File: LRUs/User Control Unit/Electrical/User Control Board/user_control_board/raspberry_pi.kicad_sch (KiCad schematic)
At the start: 2 parts, among them SW1 SW_SPDT

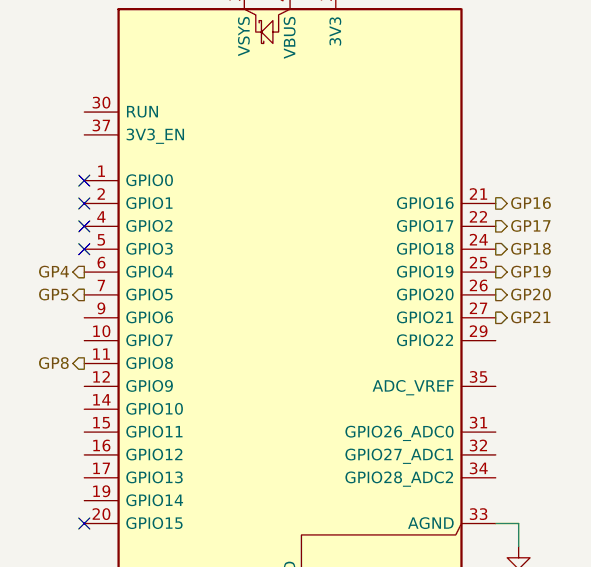
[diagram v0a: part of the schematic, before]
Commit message: DAC added Removed unnecessary modules.
Need to make custom footprint for dac.
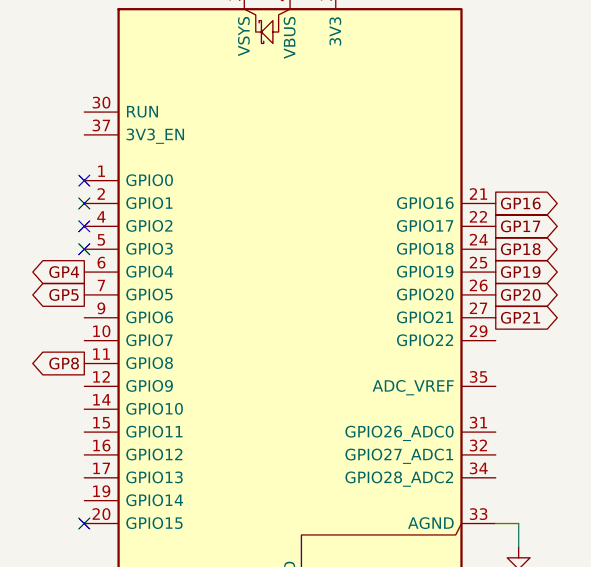
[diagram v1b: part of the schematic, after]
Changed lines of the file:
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@@
 		)
 	)
-	(hierarchical_label "GP19"
+	(global_label "GP18"
+		(shape output)
+		(at 168.91 88.9 0)
+		(fields_autoplaced yes)
+		(effects
+			(font
+				(size 1.27 1.27)
+			)
+			(justify left)
+		)
+		(property "Intersheetrefs" "${INTERSHEET_REFS}"
+			(at 176.8542 88.9 0)
+			(hide yes)
+			(show_name no)
+			(do_not_autoplace no)
+			(effects
+				(font
+					(size 1.27 1.27)
+				)
+				(justify left)
+			)
+		)
+	)
+	(global_label "GP4"
+		(shape output)
+		(at 123.19 91.44 180)
+		(fields_autoplaced yes)
+		(effects
+			(font
+				(size 1.27 1.27)
+			)
+			(justify right)
+		)
+		(property "Intersheetrefs" "${INTERSHEET_REFS}"
+			(at 116.4553 91.44 0)
+			(hide yes)
+			(show_name no)
+			(do_not_autoplace no)
+			(effects
+				(font
+					(size 1.27 1.27)
+				)
+				(justify right)
+			)
+		)
+	)
+	(global_label "GP8"
+		(shape output)
+		(at 123.19 101.6 180)
+		(fields_autoplaced yes)
+		(effects
+			(font
+				(size 1.27 1.27)
+			)
+			(justify right)
+		)
+		(property "Intersheetrefs" "${INTERSHEET_REFS}"
+			(at 116.4553 101.6 0)
+			(hide yes)
+			(show_name no)
+			(do_not_autoplace no)
+			(effects
+				(font
+					(size 1.27 1.27)
+				)
+				(justify right)
+			)
+		)
+	)
+	(global_label "GP5"
+		(shape output)
+		(at 123.19 93.98 180)
+		(fields_autoplaced yes)
+		(effects
+			(font
+				(size 1.27 1.27)
+			)
+			(justify right)
+		)
+		(property "Intersheetrefs" "${INTERSHEET_REFS}"
+			(at 116.4553 93.98 0)
+			(hide yes)
+			(show_name no)
+			(do_not_autoplace no)
+			(effects
+				(font
+					(size 1.27 1.27)
+				)
+				(justify right)
+			)
+		)
+	)
+	(global_label "GP16"
+		(shape output)
+		(at 168.91 83.82 0)
+		(fields_autoplaced yes)
+		(effects
+			(font
+				(size 1.27 1.27)
+			)
+			(justify left)
+		)
+		(property "Intersheetrefs" "${INTERSHEET_REFS}"
+			(at 176.8542 83.82 0)
+			(hide yes)
+			(show_name no)
+			(do_not_autoplace no)
+			(effects
+				(font
+					(size 1.27 1.27)
+				)
+				(justify left)
+			)
+		)
+	)
+	(global_label "GP21"
+		(shape output)
+		(at 168.91 96.52 0)
+		(fields_autoplaced yes)
+		(effects
+			(font
+				(size 1.27 1.27)
+			)
+			(justify left)
+		)
+		(property "Intersheetrefs" "${INTERSHEET_REFS}"
+			(at 176.8542 96.52 0)
+			(hide yes)
+			(show_name no)
+			(do_not_autoplace no)
+			(effects
+				(font
+					(size 1.27 1.27)
+				)
+				(justify left)
+			)
+		)
+	)
+	(global_label "GP20"
+		(shape output)
+		(at 168.91 93.98 0)
+		(fields_autoplaced yes)
+		(effects
+			(font
+				(size 1.27 1.27)
+			)
+			(justify left)
+		)
+		(property "Intersheetrefs" "${INTERSHEET_REFS}"
+			(at 176.8542 93.98 0)
+			(hide yes)
+			(show_name no)
+			(do_not_autoplace no)
+			(effects
+				(font
+					(size 1.27 1.27)
+				)
+				(justify left)
+			)
+		)
+	)
+	(global_label "GP17"
+		(shape output)
+		(at 168.91 86.36 0)
+		(fields_autoplaced yes)
+		(effects
+			(font
+				(size 1.27 1.27)
+			)
+			(justify left)
+		)
+		(property "Intersheetrefs" "${INTERSHEET_REFS}"
+			(at 176.8542 86.36 0)
+			(hide yes)
+			(show_name no)
+			(do_not_autoplace no)
+			(effects
+				(font
+					(size 1.27 1.27)
+				)
+				(justify left)
+			)
+		)
+	)
+	(global_label "GP19"
 		(shape output)
 		(at 168.91 91.44 0)
-		(effects
-			(font
-				(size 1.27 1.27)
-			)
-			(justify left)
-		)
-	)
-	(hierarchical_label "GP20"
-		(shape output)
-		(at 168.91 93.98 0)
-		(effects
-			(font
-				(size 1.27 1.27)
-			)
-			(justify left)
-		)
-	)
-	(hierarchical_label "GP21"
-		(shape output)
-		(at 168.91 96.52 0)
-		(effects
-			(font
-				(size 1.27 1.27)
-			)
-			(justify left)
-		)
-	)
-	(hierarchical_label "GP5"
-		(shape output)
-		(at 123.19 93.98 180)
-		(effects
-			(font
-				(size 1.27 1.27)
-			)
-			(justify right)
-		)
-	)
-	(hierarchical_label "GP16"
-		(shape output)
-		(at 168.91 83.82 0)
-		(effects
-			(font
-				(size 1.27 1.27)
-			)
-			(justify left)
-		)
-	)
-	(hierarchical_label "GP18"
-		(shape output)
-		(at 168.91 88.9 0)
-		(effects
-			(font
-				(size 1.27 1.27)
-			)
-			(justify left)
-		)
-	)
-	(hierarchical_label "GP17"
-		(shape output)
-		(at 168.91 86.36 0)
-		(effects
-			(font
-				(size 1.27 1.27)
-			)
-			(justify left)
-		)
-	)
-	(hierarchical_label "GP4"
-		(shape output)
-		(at 123.19 91.44 180)
-		(effects
-			(font
-				(size 1.27 1.27)
-			)
-			(justify right)
-		)
-	)
-	(hierarchical_label "GP8"
-		(shape output)
-		(at 123.19 101.6 180)
-		(effects
-			(font
-				(size 1.27 1.27)
-			)
-			(justify right)
-		)
-	)
+		(fields_autoplaced yes)
+		(effects
+			(font
+				(size 1.27 1.27)
+			)
+			(justify left)
+		)
+		(property "Intersheetrefs" "${INTERSHEET_REFS}"
+			(at 176.8542 91.44 0)
+			(hide yes)
+			(show_name no)
+			(do_not_autoplace no)
+			(effects
+				(font
+					(size 1.27 1.27)
+				)
+				(justify left)
+			)
+		)
+	)

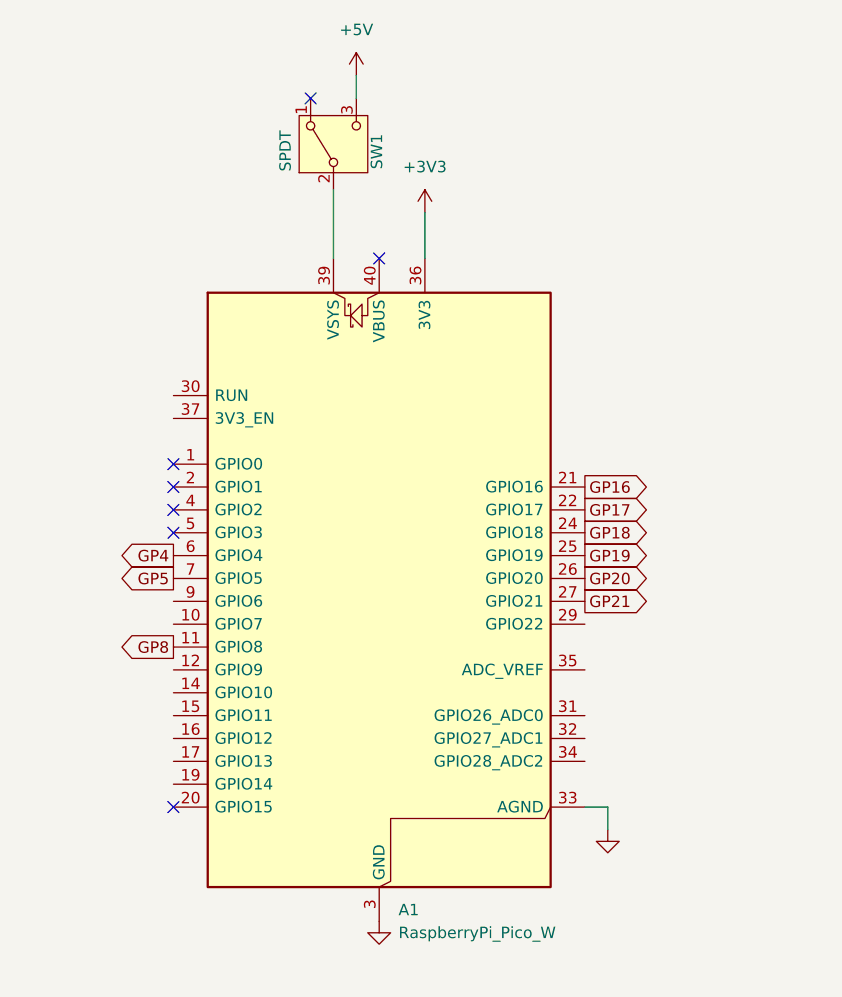
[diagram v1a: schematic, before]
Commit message: need to run DCR
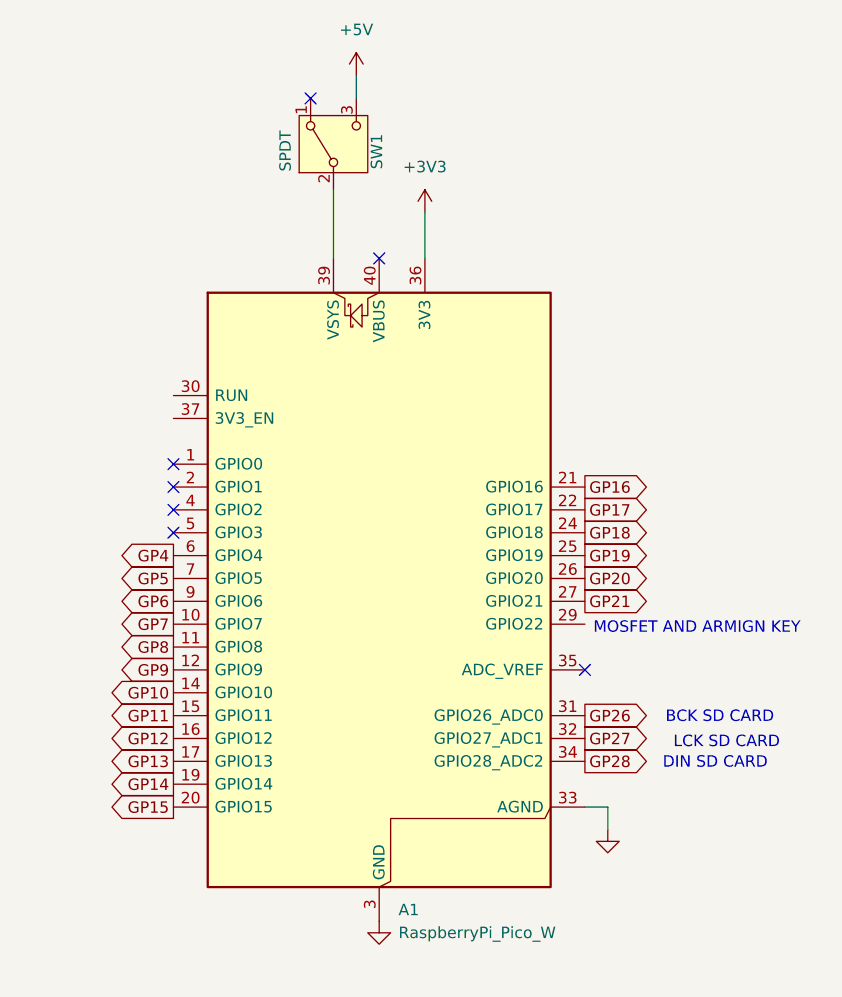
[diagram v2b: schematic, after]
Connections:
- net GP7: now reaches A1.10 (GPIO7)
- net GP9: now reaches A1.12 (GPIO9)
- net GP10: now reaches A1.14 (GPIO10)
- net GP11: now reaches A1.15 (GPIO11)
- net GP12: now reaches A1.16 (GPIO12)
- net GP13: now reaches A1.17 (GPIO13)
- net GP14: now reaches A1.19 (GPIO14)
- net GP15: now reaches A1.20 (GPIO15)
- net GP26: now reaches A1.31 (GPIO26_ADC0)
- net GP27: now reaches A1.32 (GPIO27_ADC1)
- net GP28: now reaches A1.34 (GPIO28_ADC2)
- net GP6: now reaches A1.9 (GPIO6)
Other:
- note added: "BCK SD CARD"
- note added: "DIN SD CARD"
- note added: "LCK SD CARD"
- note added: "MOSFET AND ARMIGN KEY"

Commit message: connectors and 5v buck partially done
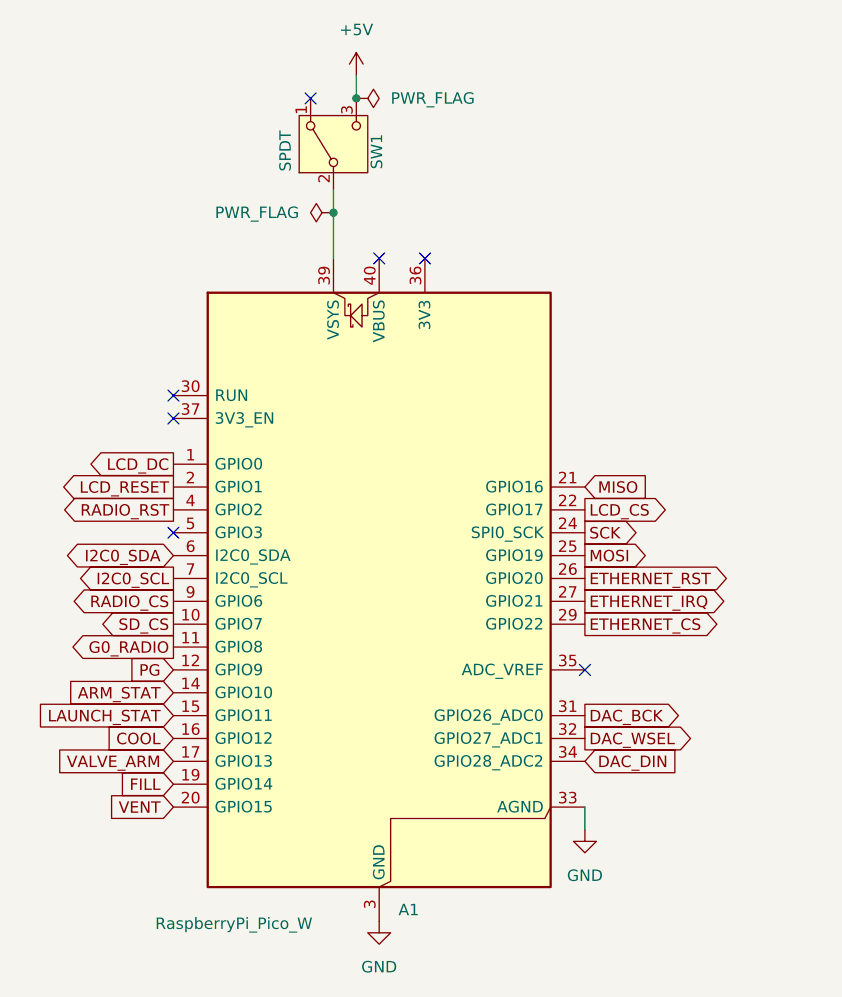
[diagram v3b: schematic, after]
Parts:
- A1: footprint Module:RaspberryPi_Pico_W_SMD_HandSolder -> Module:RaspberryPi_Pico_Common_Unspecified
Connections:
- net LCD_DC: now reaches A1.1 (GPIO0)
- net LCD_RESET: now reaches A1.2 (GPIO1)
- net ETHERNET_CS: now reaches A1.29 (GPIO22)
- net RADIO_RST: now reaches A1.4 (GPIO2)
- net +3V3: no longer names the net of A1.36 (3V3)
- net GP10 renamed ARM_STAT
- net GP11 renamed LAUNCH_STAT
- net GP12 renamed COOL
- net GP13 renamed VALVE_ARM
- net GP14 renamed FILL
- net GP15 renamed VENT
- net GP16 renamed MISO
- net GP17 renamed LCD_CS
- net GP18 renamed SCK
- net GP19 renamed MOSI
- net GP20 renamed ETHERNET_RST
- net GP21 renamed ETHERNET_IRQ
- net GP26 renamed DAC_BCK
- net GP27 renamed DAC_WSEL
- net GP28 renamed DAC_DIN
- net GP4 renamed I2C0_SDA
- net GP5 renamed I2C0_SCL
- net GP6 renamed RADIO_CS
- net GP7 renamed SD_CS
- net GP8 renamed G0_RADIO
- net GP9 renamed PG
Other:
- note removed: "BCK SD CARD"
- note removed: "DIN SD CARD"
- note removed: "LCK SD CARD"
- note removed: "MOSFET AND ARMIGN KEY"
